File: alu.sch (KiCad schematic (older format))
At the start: 280 parts, among them U1 C96ABC, U10 74ACT32, U11 74ACT86, U12 74ACT86, U13 74ACT283, U14 74ACT283, U15 74ACT253, U16 74ACT253, U17 74ACT253, U18 74ACT253, U2 74ACT04, U3 74ACT04, U4 74ACT158, U5 74ACT158, U6 74ACT158, U7 74ACT08, U8 74ACT08, U9 74ACT32

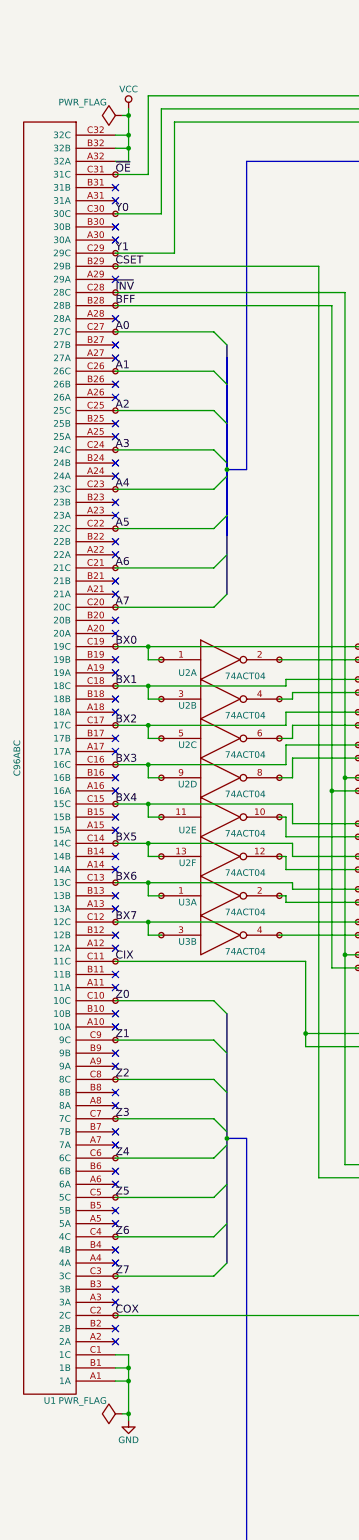
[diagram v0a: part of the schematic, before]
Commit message: pcb routing
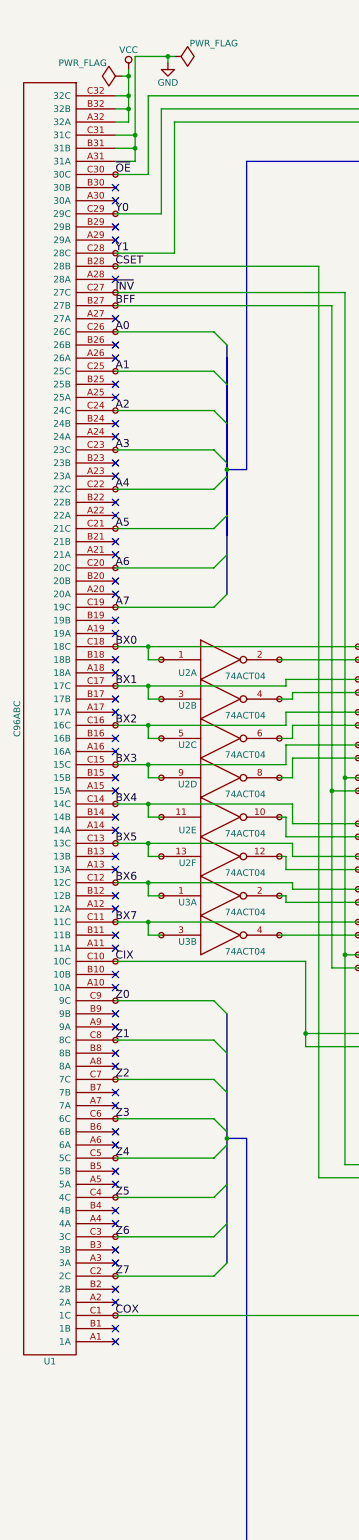
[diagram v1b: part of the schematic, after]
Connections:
- net A0: now also U1.C26 (26C); no longer U1.C27 (27C)
- net A1: now also U1.C25 (25C); no longer U1.C26 (26C)
- net A2: now also U1.C24 (24C); no longer U1.C25 (25C)
- net A3: now also U1.C23 (23C); no longer U1.C24 (24C)
- net A4: now also U1.C22 (22C); no longer U1.C23 (23C)
- net A5: now also U1.C21 (21C); no longer U1.C22 (22C)
- net A6: now also U1.C20 (20C); no longer U1.C21 (21C)
- net A7: now also U1.C19 (19C); no longer U1.C20 (20C)
- net BFF: now also U1.B27 (27B); no longer U1.B28 (28B)
- net BX0: now also U1.C18 (18C); no longer U1.C19 (19C)
- net BX1: now also U1.C17 (17C); no longer U1.C18 (18C)
- net BX2: now also U1.C16 (16C); no longer U1.C17 (17C)
- net BX3: now also U1.C15 (15C); no longer U1.C16 (16C)
- net BX4: now also U1.C14 (14C); no longer U1.C15 (15C)
- net BX5: now also U1.C13 (13C); no longer U1.C14 (14C)
- net BX6: now also U1.C12 (12C); no longer U1.C13 (13C)
- net BX7: now also U1.C11 (11C); no longer U1.C12 (12C)
- net CIX: now also U1.C10 (10C); no longer U1.C11 (11C)
- net COX: now also U1.C1 (1C); no longer U1.C2 (2C)
- net CSET: now also U1.B28 (28B); no longer U1.B29 (29B)
- net GND: now also U1.A31 (31A), U1.B31 (31B), U1.C31 (31C); no longer U1.A1 (1A), U1.B1 (1B), U1.C1 (1C)
- net Y0: now also U1.C29 (29C); no longer U1.C30 (30C)
- net Y1: now also U1.C28 (28C); no longer U1.C29 (29C)
- net Z0: now also U1.C9 (9C); no longer U1.C10 (10C)
- net Z1: now also U1.C8 (8C); no longer U1.C9 (9C)
- net Z2: now also U1.C7 (7C); no longer U1.C8 (8C)
- net Z3: now also U1.C6 (6C); no longer U1.C7 (7C)
- net Z4: now also U1.C5 (5C); no longer U1.C6 (6C)
- net Z5: now also U1.C4 (4C); no longer U1.C5 (5C)
- net Z6: now also U1.C3 (3C); no longer U1.C4 (4C)
- net Z7: now also U1.C2 (2C); no longer U1.C3 (3C)
- net ~INV: now also U1.C27 (27C); no longer U1.C28 (28C)
- net ~OE: now also U1.C30 (30C); no longer U1.C31 (31C)
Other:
- moved on the sheet: U1
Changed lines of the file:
@@
 L C96ABC U1
 U 1 1 57E75D13
-P 3900 6600
-F 0 "U1" H 3900 11500 50  0000 C CNN
-F 1 "C96ABC" V 4150 6600 50  0000 C CNN
-F 2 "Mechanical_Sockets:Socket_DIN41612-CaseC1-full-Male-96Pin-3rows" H 3900 6600 50  0001 C CNN
-F 3 "" H 3900 6600 50  0000 C CNN
-	1    3900 6600
+P 3900 6300
+F 0 "U1" H 3900 11200 50  0000 C CNN
+F 1 "C96ABC" V 4150 6300 50  0000 C CNN
+F 2 "Mechanical_Sockets:Socket_DIN41612-CaseC1-full-Male-96Pin-3rows" H 3900 6300 50  0001 C CNN
+F 3 "" H 3900 6300 50  0000 C CNN
+	1    3900 6300
 	-1   0    0    1
 $EndComp
@@
 L VCC #PWR01
 U 1 1 57E80CD3
-P 4500 1650
-F 0 "#PWR01" H 4500 1500 50  0001 C CNN
-F 1 "VCC" H 4500 1800 50  0000 C CNN
-F 2 "" H 4500 1650 50  0000 C CNN
-F 3 "" H 4500 1650 50  0000 C CNN
-	1    4500 1650
+P 4500 1350
+F 0 "#PWR01" H 4500 1200 50  0001 C CNN
+F 1 "VCC" H 4500 1500 50  0000 C CNN
+F 2 "" H 4500 1350 50  0000 C CNN
+F 3 "" H 4500 1350 50  0000 C CNN
+	1    4500 1350
 	1    0    0    -1
 $EndComp
@@
 L GND #PWR02
 U 1 1 57E812B2
-P 4500 11650
-F 0 "#PWR02" H 4500 11400 50  0001 C CNN
-F 1 "GND" H 4500 11500 50  0000 C CNN
-F 2 "" H 4500 11650 50  0000 C CNN
-F 3 "" H 4500 11650 50  0000 C CNN
-	1    4500 11650
-	1    0    0    -1
+P 4800 1300
+F 0 "#PWR02" H 4800 1050 50  0001 C CNN
+F 1 "GND" H 4800 1150 50  0000 C CNN
+F 2 "" H 4800 1300 50  0000 C CNN
+F 3 "" H 4800 1300 50  0000 C CNN
+	1    4800 1300
+	-1   0    0    -1
 $EndComp
 $Comp
@@
 L PWR_FLAG #FLG04
 U 1 1 57E9C81D
-P 4450 1700
-F 0 "#FLG04" H 4450 1795 50  0001 C CNN
-F 1 "PWR_FLAG" V 4550 2000 50  0000 C CNN
-F 2 "" H 4450 1700 50  0000 C CNN
-F 3 "" H 4450 1700 50  0000 C CNN
-	1    4450 1700
+P 4450 1400
+F 0 "#FLG04" H 4450 1495 50  0001 C CNN
+F 1 "PWR_FLAG" V 4550 1700 50  0000 C CNN
+F 2 "" H 4450 1400 50  0000 C CNN
+F 3 "" H 4450 1400 50  0000 C CNN
+	1    4450 1400
 	0    -1   -1   0
 $EndComp
@@
 L PWR_FLAG #FLG05
 U 1 1 57E410D7
-P 4450 11600
-F 0 "#FLG05" H 4450 11695 50  0001 C CNN
-F 1 "PWR_FLAG" V 4550 11900 50  0000 C CNN
-F 2 "" H 4450 11600 50  0000 C CNN
-F 3 "" H 4450 11600 50  0000 C CNN
-	1    4450 11600
-	0    -1   -1   0
+P 4850 1250
+F 0 "#FLG05" H 4850 1345 50  0001 C CNN
+F 1 "PWR_FLAG" V 4950 1550 50  0000 C CNN
+F 2 "" H 4850 1250 50  0000 C CNN
+F 3 "" H 4850 1250 50  0000 C CNN
+	1    4850 1250
+	0    1    -1   0
 $EndComp
 Wire Wire Line
@@
 	4650 2150 4400 2150
 Wire Wire Line
-	4500 1850 4400 1850
-Wire Wire Line
-	4500 1650 4500 2050
-Wire Wire Line
-	4500 1950 4400 1950
-Connection ~ 4500 1850
-Wire Wire Line
-	4500 2050 4400 2050
-Connection ~ 4500 1950
+	4500 1550 4400 1550
 Wire Wire Line
-	4400 11150 4500 11150
+	4500 1350 4500 1750
 Wire Wire Line
-	4500 11150 4500 11650
+	4500 1650 4400 1650
+Connection ~ 4500 1550
 Wire Wire Line
-	4400 11250 4500 11250
-Connection ~ 4500 11250
+	4500 1750 4400 1750
+Connection ~ 4500 1650
 Wire Wire Line
-	4400 11350 4500 11350
-Connection ~ 4500 11350
+	4800 1250 4800 1300
 Wire Wire Line
 	5650 5850 6250 5850
@@
 Connection ~ 7650 9550
 Wire Wire Line
-	4450 1700 4500 1700
-Connection ~ 4500 1700
+	4450 1400 4500 1400
+Connection ~ 4500 1400
 Wire Wire Line
 	8000 10100 7650 10100
@@
 Connection ~ 7650 10450
 Wire Wire Line
-	4500 11600 4450 11600
-Connection ~ 4500 11600
+	4550 1250 4850 1250
+Connection ~ 4800 1250
 $Comp
 L C C9
@@
 	1    0    0    -1
 $EndComp
+Wire Wire Line
+	4400 1950 4550 1950
+Wire Wire Line
+	4550 1250 4550 2050
+Wire Wire Line
+	4400 1850 4550 1850
+Connection ~ 4550 1850
+Wire Wire Line
+	4550 2050 4400 2050
+Connection ~ 4550 1950
 $EndSCHEMATC
